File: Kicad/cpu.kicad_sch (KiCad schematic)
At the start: 7 parts, among them U1 8086_Min_Mode, U10 74HCT573, U11 74HCT245, U4 74HCT138, U7 74HCT573, U8 74HCT245, U9 74HCT573

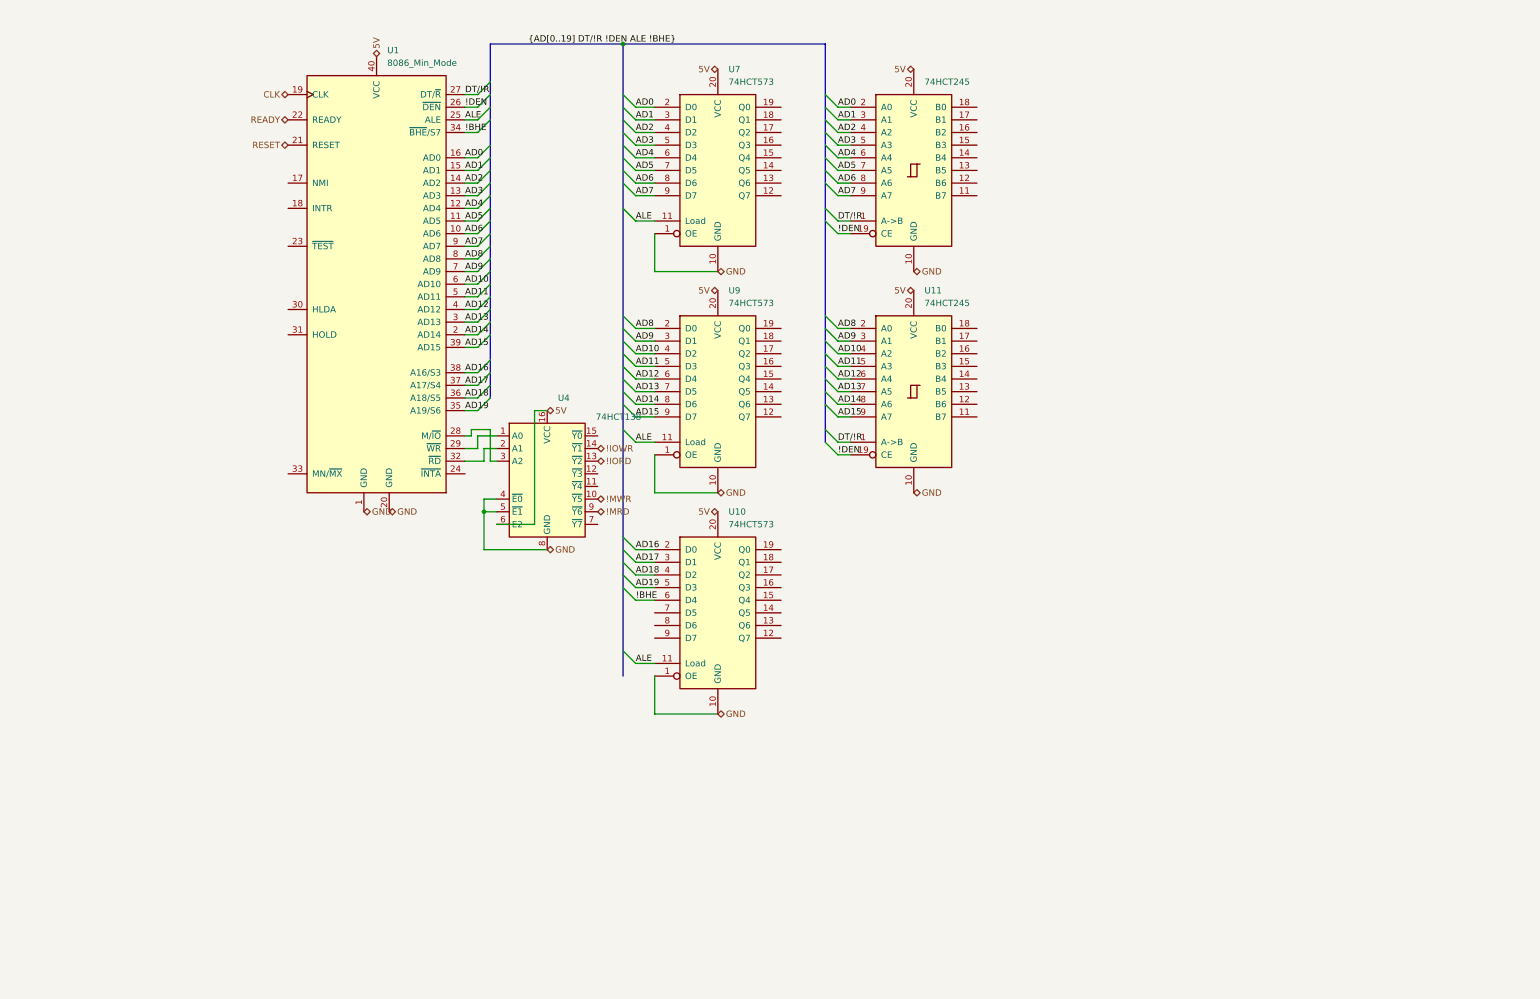
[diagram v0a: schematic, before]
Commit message: Add files via upload
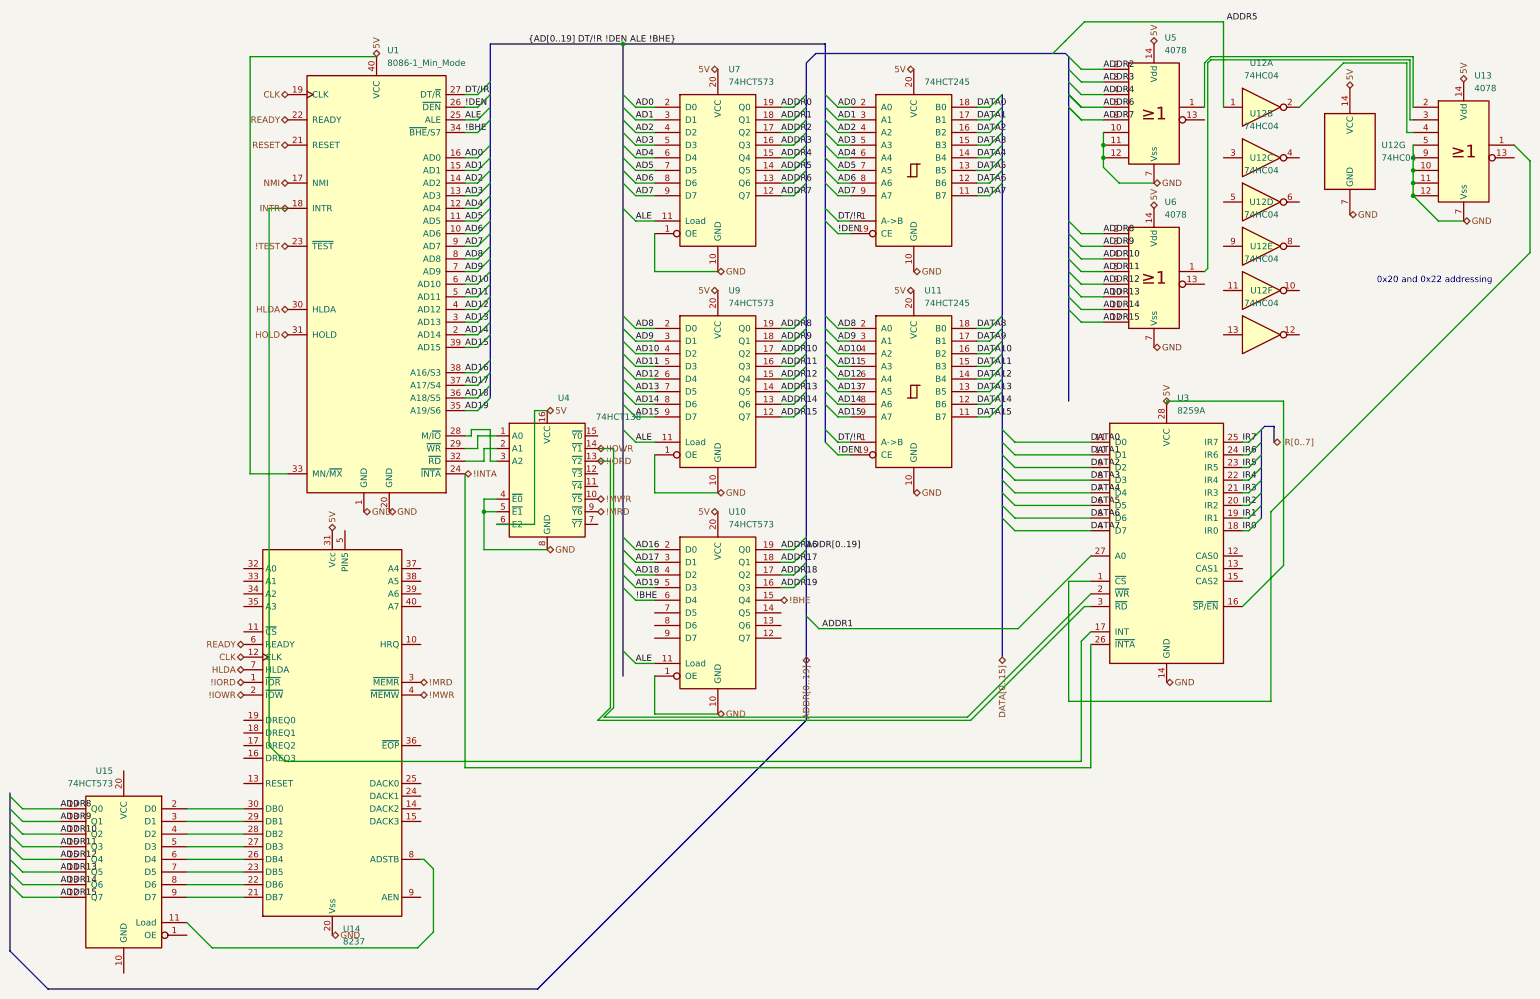
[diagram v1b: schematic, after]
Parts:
- added U12: 74HC04, symbol 74xx:74HC04
- added U13, U5, U6: 4078, symbol 4xxx_IEEE:4078
- added U14: 8237, Package_DIP:DIP-40_W15.24mm, symbol Interface:8237
- added U15: 74HCT573, Package_DIP:DIP-20_W7.62mm, symbol 74xx:74LS573
- added U3: 8259A, Package_DIP:DIP-28_W15.24mm, symbol Interface:8259A
- U1: value 8086_Min_Mode -> 8086-1_Min_Mode
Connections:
- net !BHE: now also U10.15 (Q4)
- net !IORD: now also U14.1 (~{IOR}), U3.3 (~{RD})
- net !IOWR: now also U14.2 (~{IOW}), U3.2 (~{WR})
- net !MRD: now also U14.3 (~{MEMR})
- net !MWR: now also U14.4 (~{MEMW})
- net 5V: now also U1.33 (MN/~{MX}), U12.14 (VCC), U13.14 (Vdd), U14.31 (Vcc), U3.16 (~{SP}/~{EN}), U3.28 (VCC), U5.14 (Vdd), U6.14 (Vdd)
- net CLK: now also U14.12 (CLK)
- net GND: now also U12.7 (GND), U13.10, U13.11, U13.12, U13.5, U13.7 (Vss), U13.9, U14.20 (Vss), U3.14 (GND), U5.10, U5.11, U5.12, U5.7 (Vss), U6.7 (Vss)
- net READY: now also U14.6 (READY)
- net DATA15: now reaches U11.11 (B7)
- net DATA14: now reaches U11.12 (B6)
- net DATA13: now reaches U11.13 (B5)
- net DATA12: now reaches U11.14 (B4)
- net DATA11: now reaches U11.15 (B3)
- net DATA10: now reaches U11.16 (B2)
- net DATA9: now reaches U11.17 (B1)
- net DATA8: now reaches U11.18 (B0)
- net ADDR19: now reaches U10.16 (Q3)
- net ADDR18: now reaches U10.17 (Q2)
- net ADDR17: now reaches U10.18 (Q1)
- net ADDR16: now reaches U10.19 (Q0)
- net ADDR7: now reaches U7.12 (Q7)
- net ADDR7: now also U5.9
- net ADDR6: now reaches U7.13 (Q6)
- net ADDR6: now also U5.5
- net ADDR5: now reaches U7.14 (Q5)
- net ADDR4: now reaches U7.15 (Q4)
- net ADDR4: now also U5.4
- net ADDR3: now reaches U7.16 (Q3)
- net ADDR3: now also U5.3
- net ADDR2: now reaches U7.17 (Q2)
- net ADDR2: now also U5.2
- net ADDR1: now reaches U7.18 (Q1)
- net ADDR1: now also U3.27 (A0)
- net ADDR0: now reaches U7.19 (Q0)
- net DATA7: now reaches U8.11 (B7)
- net DATA7: now also U3.4 (D7)
- net DATA6: now reaches U8.12 (B6)
- net DATA6: now also U3.5 (D6)
- net DATA5: now reaches U8.13 (B5)
- net DATA5: now also U3.6 (D5)
- net DATA4: now reaches U8.14 (B4)
- net DATA4: now also U3.7 (D4)
- net DATA3: now reaches U8.15 (B3)
- net DATA3: now also U3.8 (D3)
- net DATA2: now reaches U8.16 (B2)
- net DATA2: now also U3.9 (D2)
- net DATA1: now reaches U8.17 (B1)
- net DATA1: now also U3.10 (D1)
- net DATA0: now reaches U8.18 (B0)
- net DATA0: now also U3.11 (D0)
- net NMI: now reaches U1.17 (NMI)
- net INTR: now reaches U1.18 (INTR)
- net INTR: now also U3.17 (INT)
- net !TEST: now reaches U1.23 (~{TEST})
- net !INTA: now reaches U1.24 (~{INTA})
- net !INTA: now also U3.26 (~{INTA})
- net HLDA: now reaches U1.30 (HLDA)
- net HLDA: now also U14.7 (HLDA)
- net HOLD: now reaches U1.31 (HOLD)
- net ADDR15: now reaches U9.12 (Q7)
- net ADDR15: now also U15.12 (Q7), U6.12
- net ADDR14: now reaches U9.13 (Q6)
- net ADDR14: now also U15.13 (Q6), U6.11
- net ADDR13: now reaches U9.14 (Q5)
- net ADDR13: now also U15.14 (Q5), U6.10
- net ADDR12: now reaches U9.15 (Q4)
- net ADDR12: now also U15.15 (Q4), U6.9
- net ADDR11: now reaches U9.16 (Q3)
- net ADDR11: now also U15.16 (Q3), U6.5
- net ADDR10: now reaches U9.17 (Q2)
- net ADDR10: now also U15.17 (Q2), U6.4
- net ADDR9: now reaches U9.18 (Q1)
- net ADDR9: now also U15.18 (Q1), U6.3
- net ADDR8: now reaches U9.19 (Q0)
- net ADDR8: now also U15.19 (Q0), U6.2
- new net: U13.1, U3.1 (~{CS})
- new net: U12.2, U13.4
- new net: U13.3, U6.1
- new net: U14.8 (ADSTB), U15.11 (Load)
- new net: U14.30 (DB0), U15.2 (D0)
- new net: U14.29 (DB1), U15.3 (D1)
- new net: U14.28 (DB2), U15.4 (D2)
- new net: U14.27 (DB3), U15.5 (D3)
- new net: U14.26 (DB4), U15.6 (D4)
- new net: U14.23 (DB5), U15.7 (D5)
- new net: U14.22 (DB6), U15.8 (D6)
- new net: U14.21 (DB7), U15.9 (D7)
- new net: U13.2, U5.1
- new net IR0: U3.18 (IR0)
- new net IR1: U3.19 (IR1)
- new net IR2: U3.20 (IR2)
- new net IR3: U3.21 (IR3)
- new net IR4: U3.22 (IR4)
- new net IR5: U3.23 (IR5)
- new net IR6: U3.24 (IR6)
- new net IR7: U3.25 (IR7)
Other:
- note added: "0x20 and 0x22 addressing"
